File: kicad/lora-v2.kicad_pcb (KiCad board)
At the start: 4 copper layers, 82.5 x 47.5 mm, 63 parts, among them J1 USB_C_Receptacle_USB2.0_16P, SW1 bootsl, SW2 reset, U1 RP2040, U2 SX1262IMLTRT, U3 4259-63, U4 AP2112K-3.3TRG1, U5 W25Q16JVSS, Y1 32MHz, Y2 12MHz

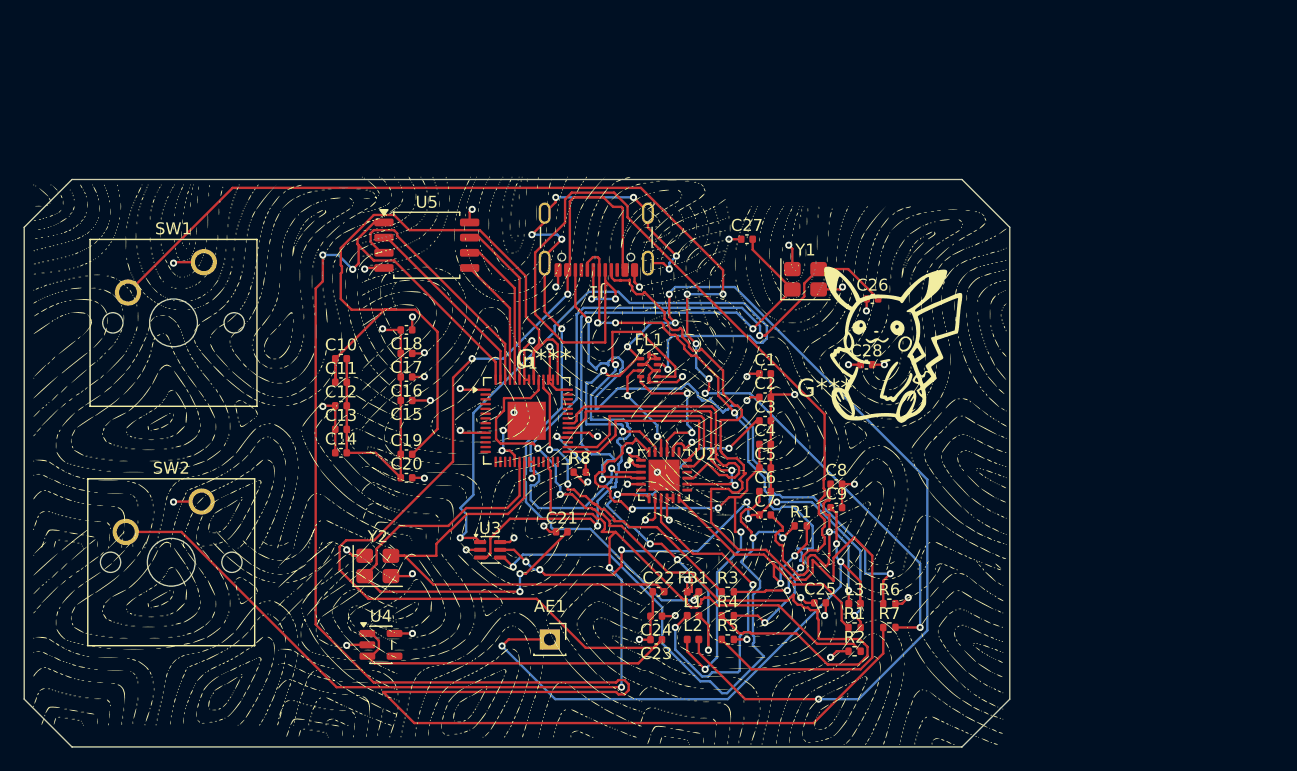
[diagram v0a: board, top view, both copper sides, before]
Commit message: Added
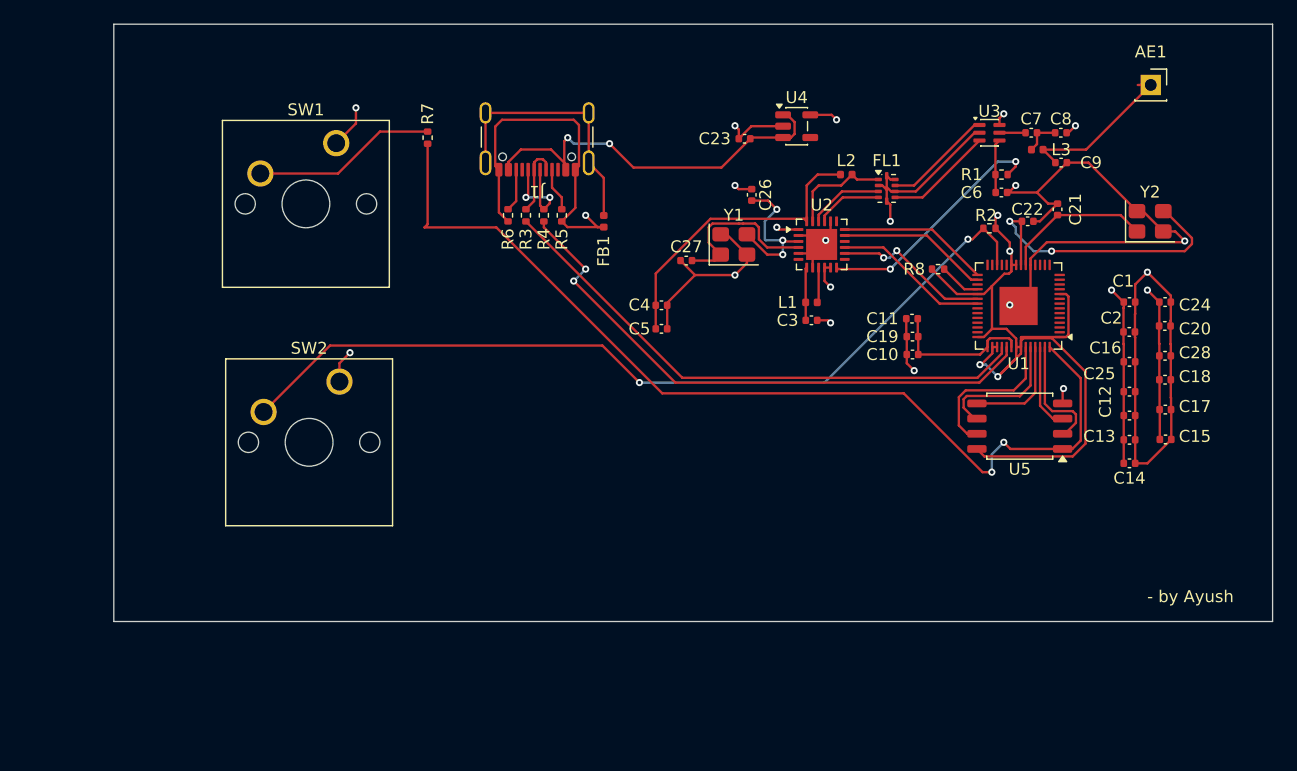
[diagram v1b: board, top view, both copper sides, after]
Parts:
- removed . (x2), G*** (x8): LOGO, LOGO
- removed the R1 at (175.5, 90.5)
- removed the R1 at (180.0, 99.0)
- added R1: 100, Resistor_SMD:R_0402_1005Metric, F.Cu at (192.3, 61.1)
- moved Y2 70.8 mm to (204.8, 65.0)
- moved AE1 68.4 mm to (204.8, 53.6)
- moved C13 66.0 mm to (203.0, 83.3)
- moved C14 66.0 mm to (203.0, 85.3)
- moved C12 66.0 mm to (203.0, 81.3)
- moved C20 64.7 mm to (206.0, 73.8), turned to 180 degrees
- moved C17 63.7 mm to (206.0, 80.8), turned to 0 degrees
- moved C18 63.6 mm to (206.0, 78.3), turned to 0 degrees
- moved C15 63.6 mm to (206.0, 83.3), turned to 0 degrees
- moved C16 60.5 mm to (203.0, 76.8), turned to 0 degrees
- moved R7 56.3 mm to (144.3, 58.0), turned to 90 degrees
- moved U4 55.6 mm to (175.2, 57.0)
- moved U3 54.5 mm to (191.3, 57.6)
- moved U5 51.9 mm to (193.8, 82.2), turned to 180 degrees
- moved C24 50.1 mm to (206.0, 71.8), turned to 0 degrees
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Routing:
- net Earth: track 394.6 -> 169.1 mm, vias 32 -> 16
- net +3V3: track 285.9 -> 112.5 mm, vias 24 -> 10
- net Net-(R7-Pad2): track 101.9 -> 15.5 mm, vias 6 -> 0
- net /SX_RFO: track 91.0 -> 8.76 mm, vias 6 -> 0
- net VBUS: track 110.7 -> 32.6 mm
- net /USB_DM: track 81.8 -> 6.03 mm, vias 4 -> 0
- net Net-(J1-CC1): track 78.1 -> 3.65 mm
- net /QSPI_SS: track 154.0 -> 81.9 mm
- net +1V1: track 71.3 -> 12.3 mm
- net Net-(J1-CC2): track 56.7 -> 3.59 mm, vias 2 -> 0
- net Net-(U3-CTRL): track 52.2 -> 4.50 mm, vias 3 -> 0
- net /SX_XTA: track 60.7 -> 13.1 mm, vias 2 -> 3
- net /RF1: track 56.7 -> 9.16 mm, vias 2 -> 0
- net Net-(J1-SHIELD): track 65.9 -> 21.9 mm, vias 8 -> 0
- net Net-(U3-RFC): track 44.9 -> 2.18 mm, vias 7 -> 0
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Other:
- board size 82.5 x 47.5 mm -> 97 x 50 mm
- board text added: "- by Ayush"
